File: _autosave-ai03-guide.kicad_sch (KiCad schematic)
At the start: 24 parts, among them SW1 SW_Push, Y1 16MHz

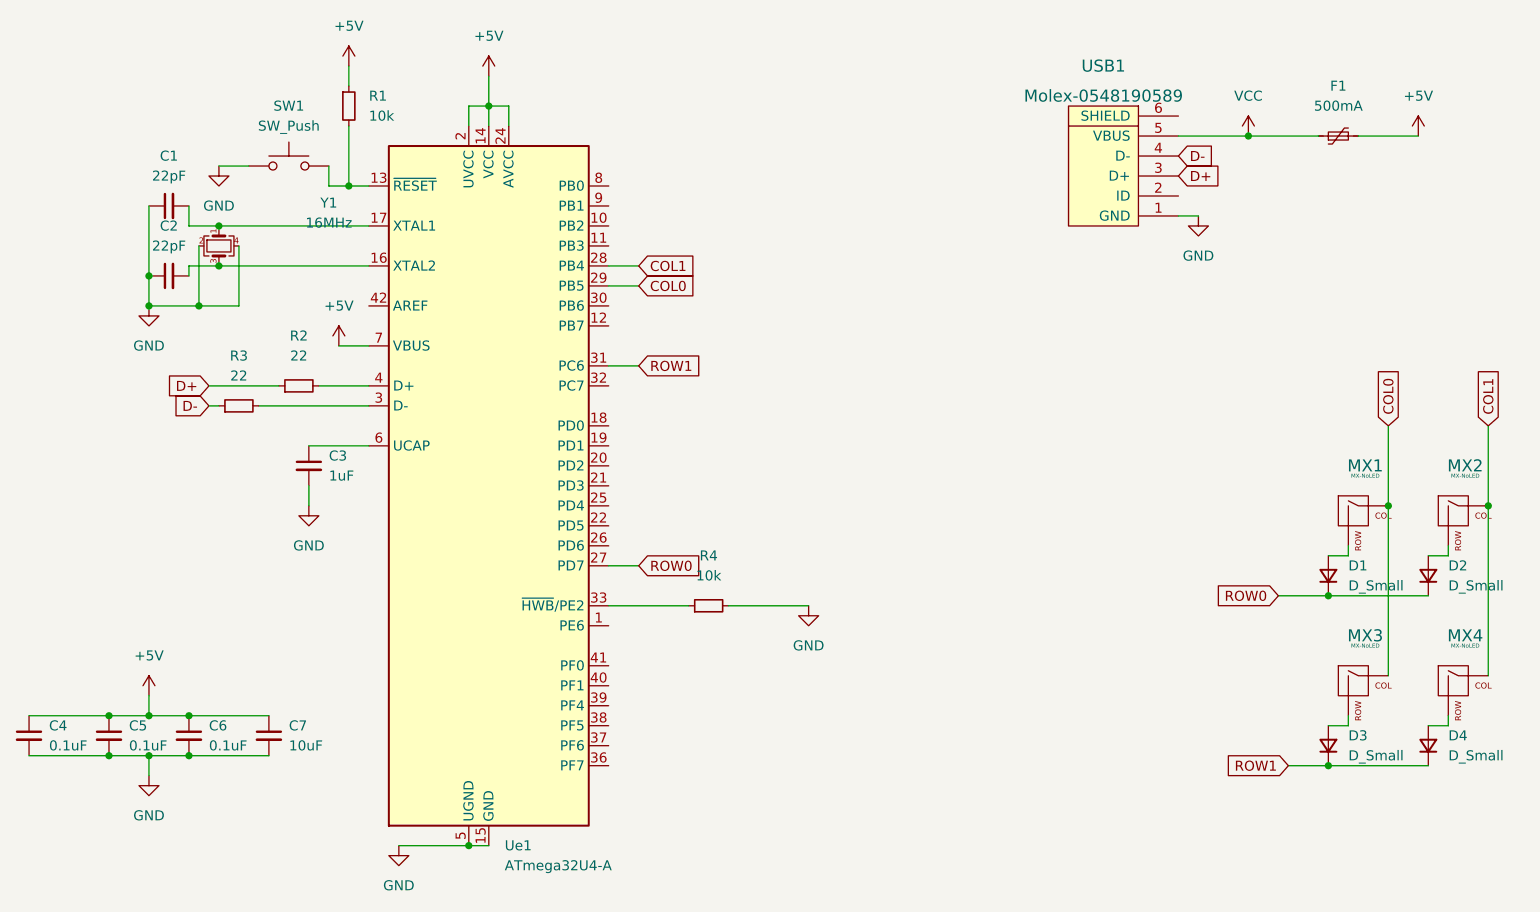
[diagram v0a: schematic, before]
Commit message: Prototype Done
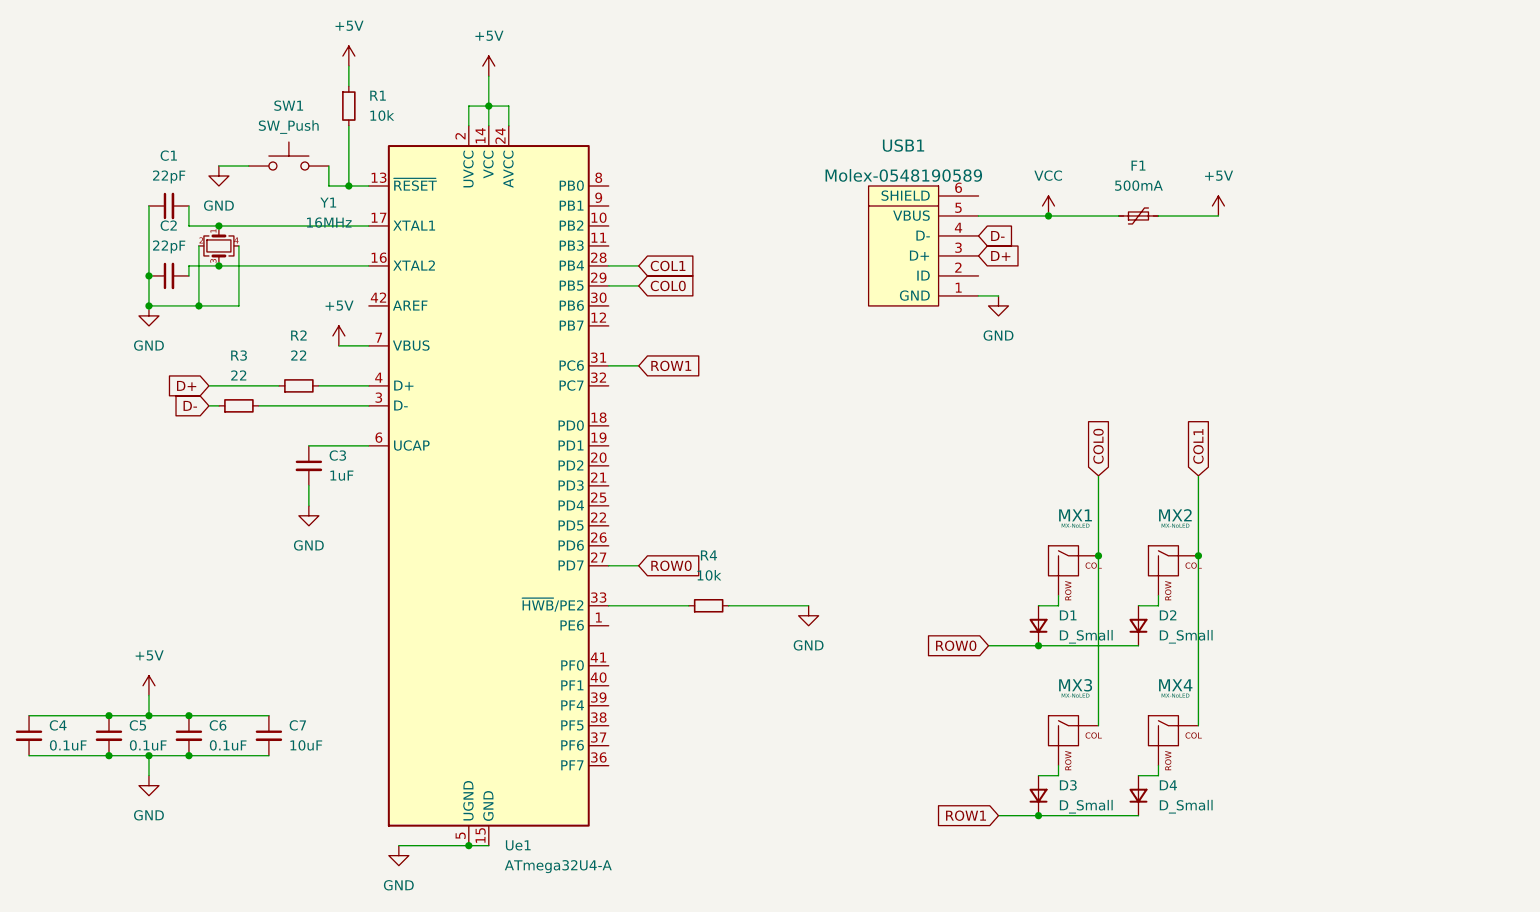
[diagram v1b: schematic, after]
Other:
- moved on the sheet: D1, D2, D3, D4, F1, MX1, MX2, MX3, MX4, USB1
